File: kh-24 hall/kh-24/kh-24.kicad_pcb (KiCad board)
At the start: 4 copper layers, 133.3 x 156 mm, 82 parts, among them CN3 Pogo Pin Receptor Right, J1 Conn_01x06, Q1 AO3401A, Q3 AO3401A, U1 SLSS49E-3, U10 SLSS49E-3, U11 H3V3U10B, U12 SLSS49E-3, U13 SLSS49E-3, U14 SLSS49E-3, U15 SLSS49E-3, U16 SLSS49E-3, U17 SLSS49E-3, U18 CD4051BM96, U19 SLSS49E-3, U2 ATtiny1616-M, U20 SLSS49E-3, U21 SLSS49E-3, U22 LM66200DRLR, U24 SLSS49E-3, U25 SLSS49E-3, U26 CD4051BM96, U27 SLSS49E-3, U28 SLSS49E-3, U29 SLSS49E-3, U3 CD4051BM96, U30 SLSS49E-3, U31 SLSS49E-3, U32 SLSS49E-3, U33 SLSS49E-3, U34 CD4051BM96, U35 SLSS49E-3, U4 SLSS49E-3, U5 H3V3U10B, U6 SLSS49E-3, U7 Pogo Pin Left, U8 AP2112K-3.3, U9 SLSS49E-3

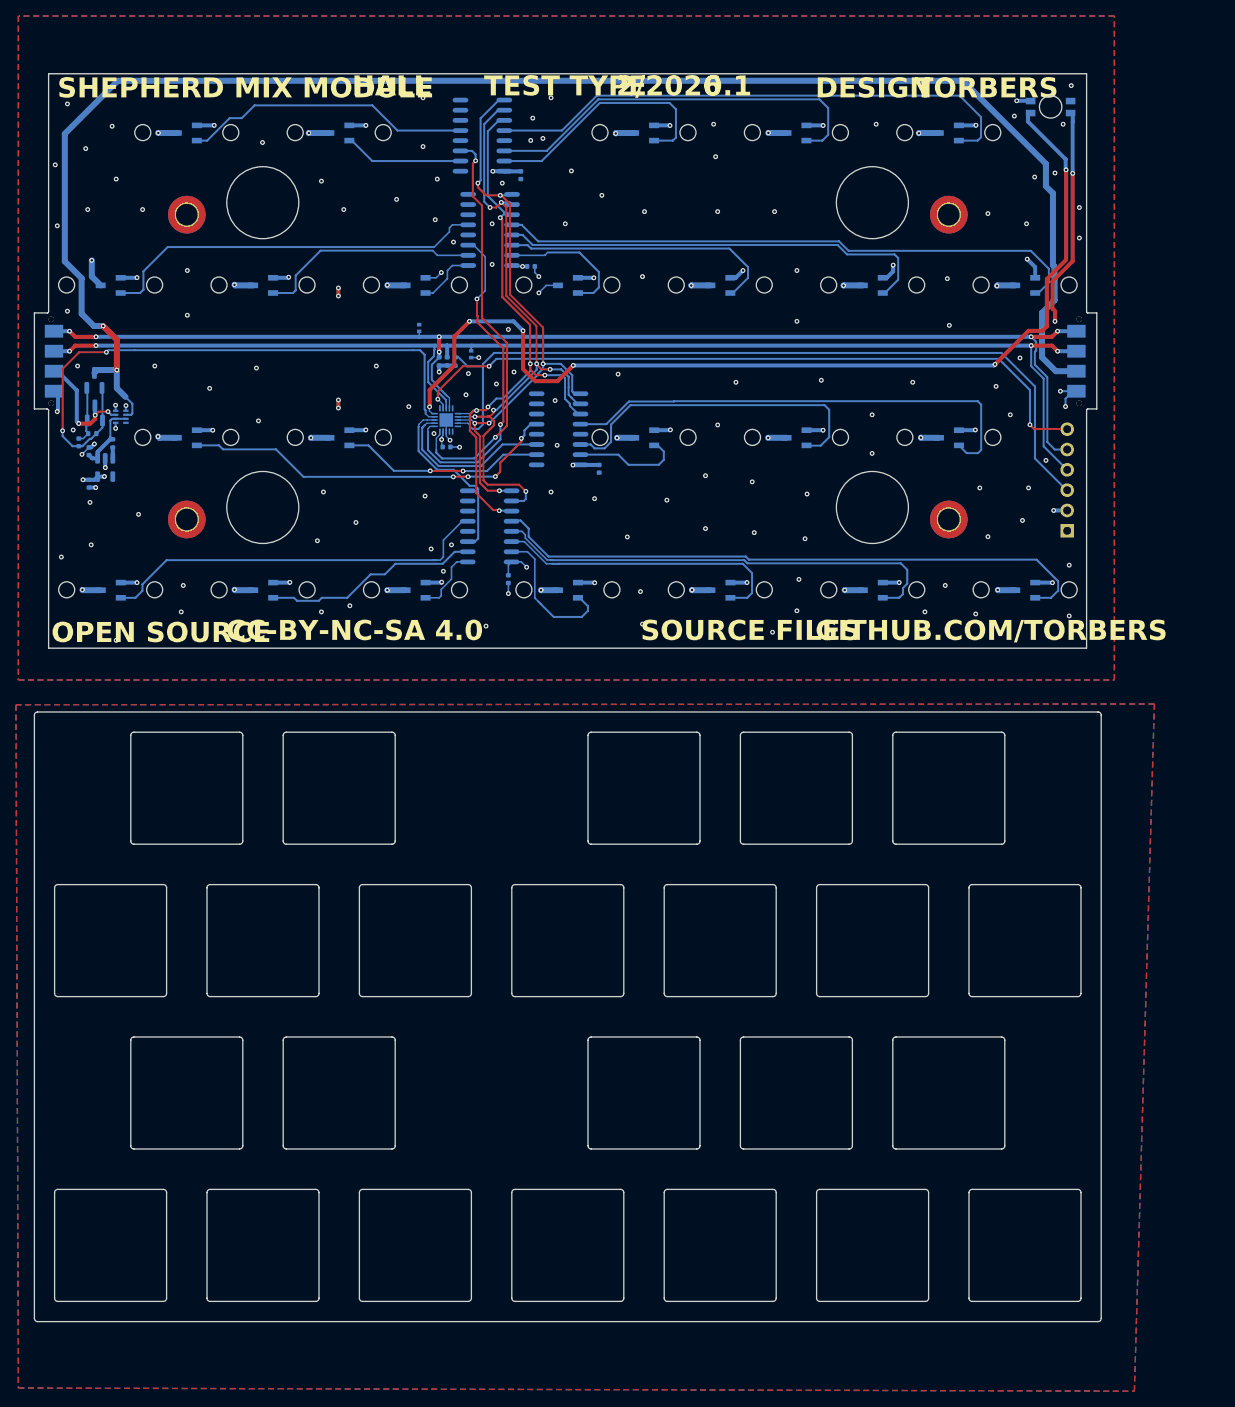
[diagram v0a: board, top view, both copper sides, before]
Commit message: prod
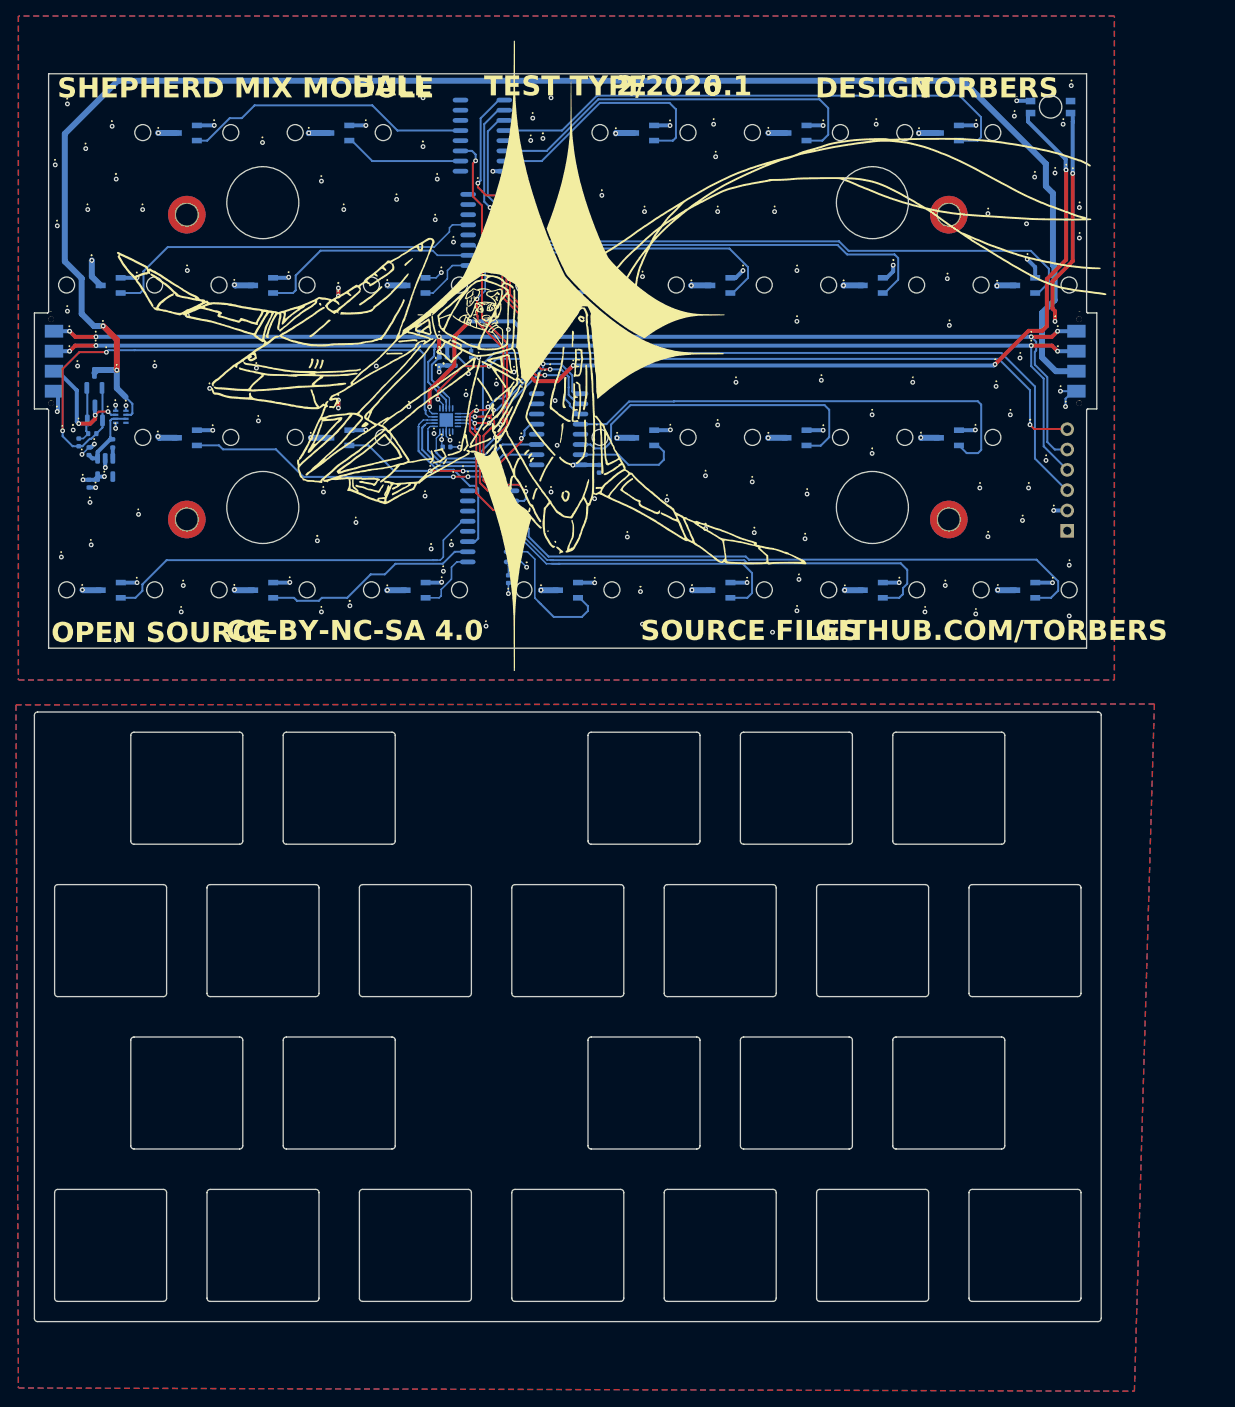
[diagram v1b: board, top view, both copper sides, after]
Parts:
- added G***: LOGO, LOGO, F.Cu at (86.6, 62.5)
